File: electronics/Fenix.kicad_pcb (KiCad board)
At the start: 2 copper layers, 130.5 x 64 mm, 24 parts, among them J1 Radio 3.5mm, J2 Relay_Control, J3 Radio 2.5mm, J3_ADR1 Conn_01x02_Pin, J4 PWR_MON, J4_LORA_PWR1 Conn_01x02_Pin, J4_SRV_EN1 Conn_01x02_Pin, J5 PWR_IN, Q1 BC548

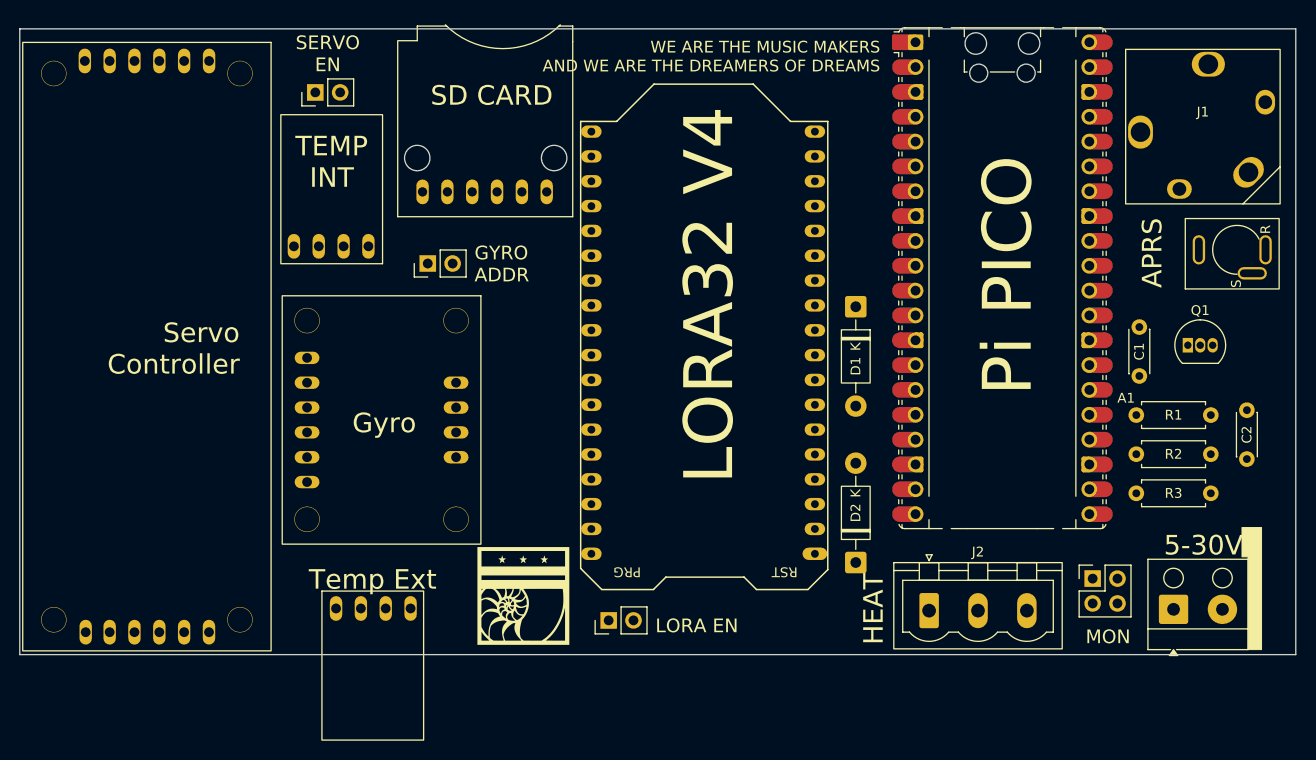
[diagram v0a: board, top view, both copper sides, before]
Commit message: Completed PCB Design
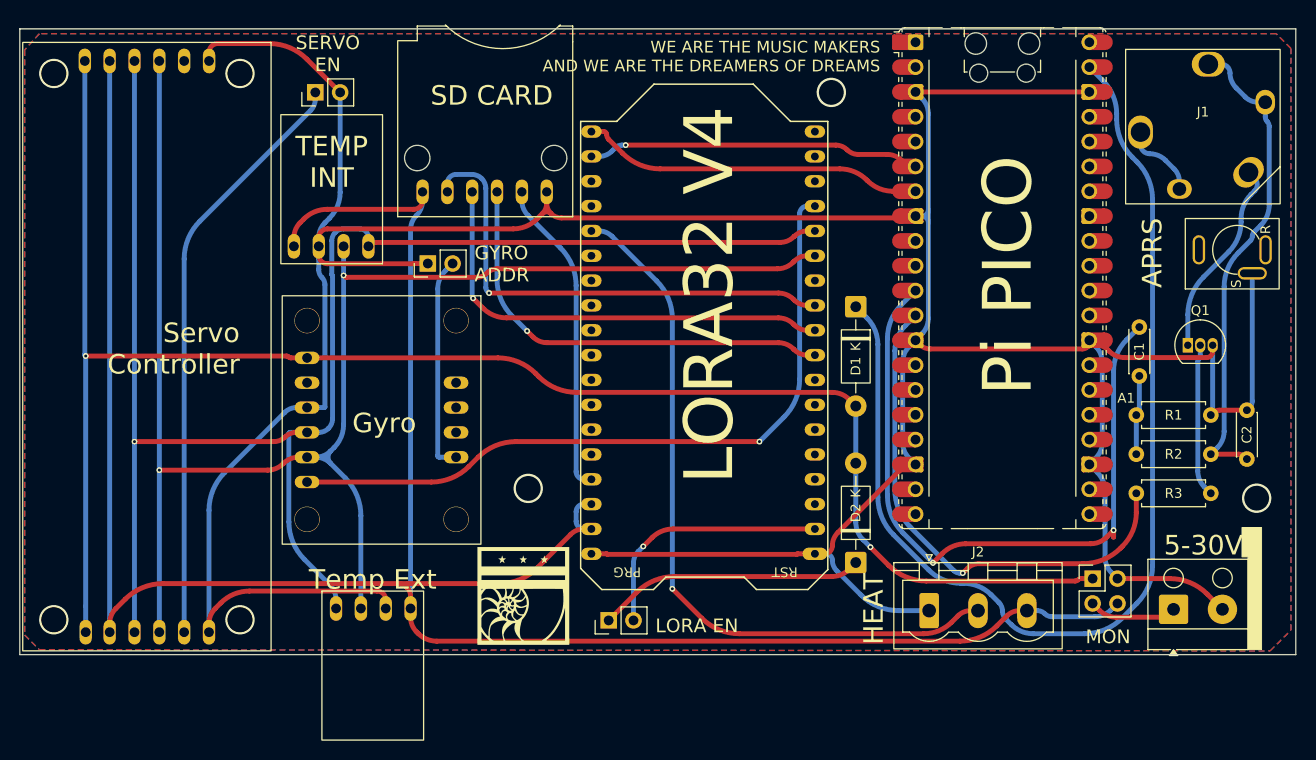
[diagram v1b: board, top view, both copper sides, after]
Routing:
- net GND: track 0.00 -> 393.0 mm, vias 0 -> 7
- net +3V3: track 0.00 -> 256.9 mm
- net +5V: track 0.00 -> 177.5 mm, vias 0 -> 2
- net /I2C_DATA: track 0.00 -> 171.2 mm, vias 0 -> 1
- net /I2C_CLK: track 0.00 -> 165.5 mm, vias 0 -> 2
- net Net-(A1-VSYS): track 0.00 -> 112.5 mm
- net Net-(A1-GPIO8): track 0.00 -> 75.5 mm, vias 0 -> 2
- net /RELAY_EN: track 0.00 -> 74.2 mm, vias 0 -> 1
- net /GYRO_RST: track 0.00 -> 74.2 mm, vias 0 -> 1
- net Net-(J4_SRV_EN1-Pin_1): track 0.00 -> 60.4 mm
- net Net-(A1-GPIO9): track 0.00 -> 53.7 mm, vias 0 -> 1
- net /SPI_CS_SD: track 0.00 -> 50.6 mm, vias 0 -> 1
- net Net-(C2-Pad1): track 0.00 -> 49.7 mm
- net /SPI_PICO: track 0.00 -> 46.9 mm, vias 0 -> 1
- net /SPI_CLK: track 0.00 -> 45.4 mm, vias 0 -> 1
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- added copper zone on B.Cu, net GND
- added copper zone on F.Cu, net GND
